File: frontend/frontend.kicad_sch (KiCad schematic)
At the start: 60 parts, among them Q1 T2N7002AK,LM, Q2 NX3008PBK,215, Q3 NX3008PBK,215, Q4 T2N7002AK,LM, Q5 NX3008PBK,215, Q6 T2N7002AK,LM, U1 ADS1291/2, U2 KC2016Z2

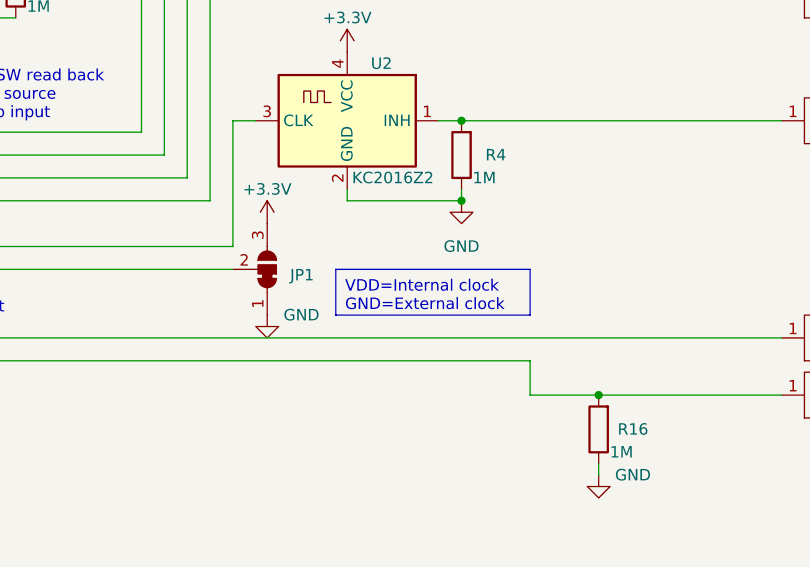
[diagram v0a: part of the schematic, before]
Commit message: Update to kicad 9
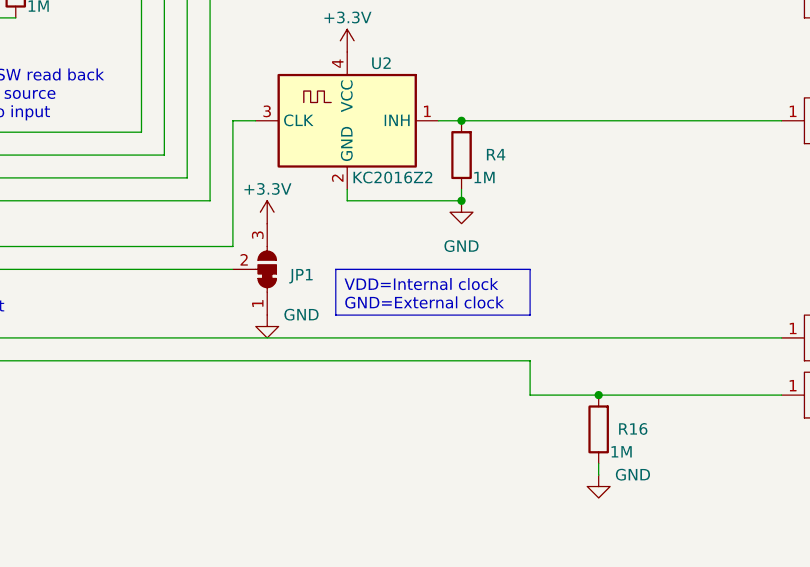
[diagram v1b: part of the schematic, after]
